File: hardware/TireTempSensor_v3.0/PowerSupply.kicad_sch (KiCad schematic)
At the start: 43 parts, among them IC3 TPS54202HDDCR, IC4 TPS54202HDDCR, Q1 FQT3P20TF, T10 TP_+5V, T11 TP_+5V, T12 TP_+5V, T13 TP_+5V, T14 TP_+3.3V, T15 TP_+2.6V, T8 TP_VCC, U2 MIC5306-2.6YD5-TR

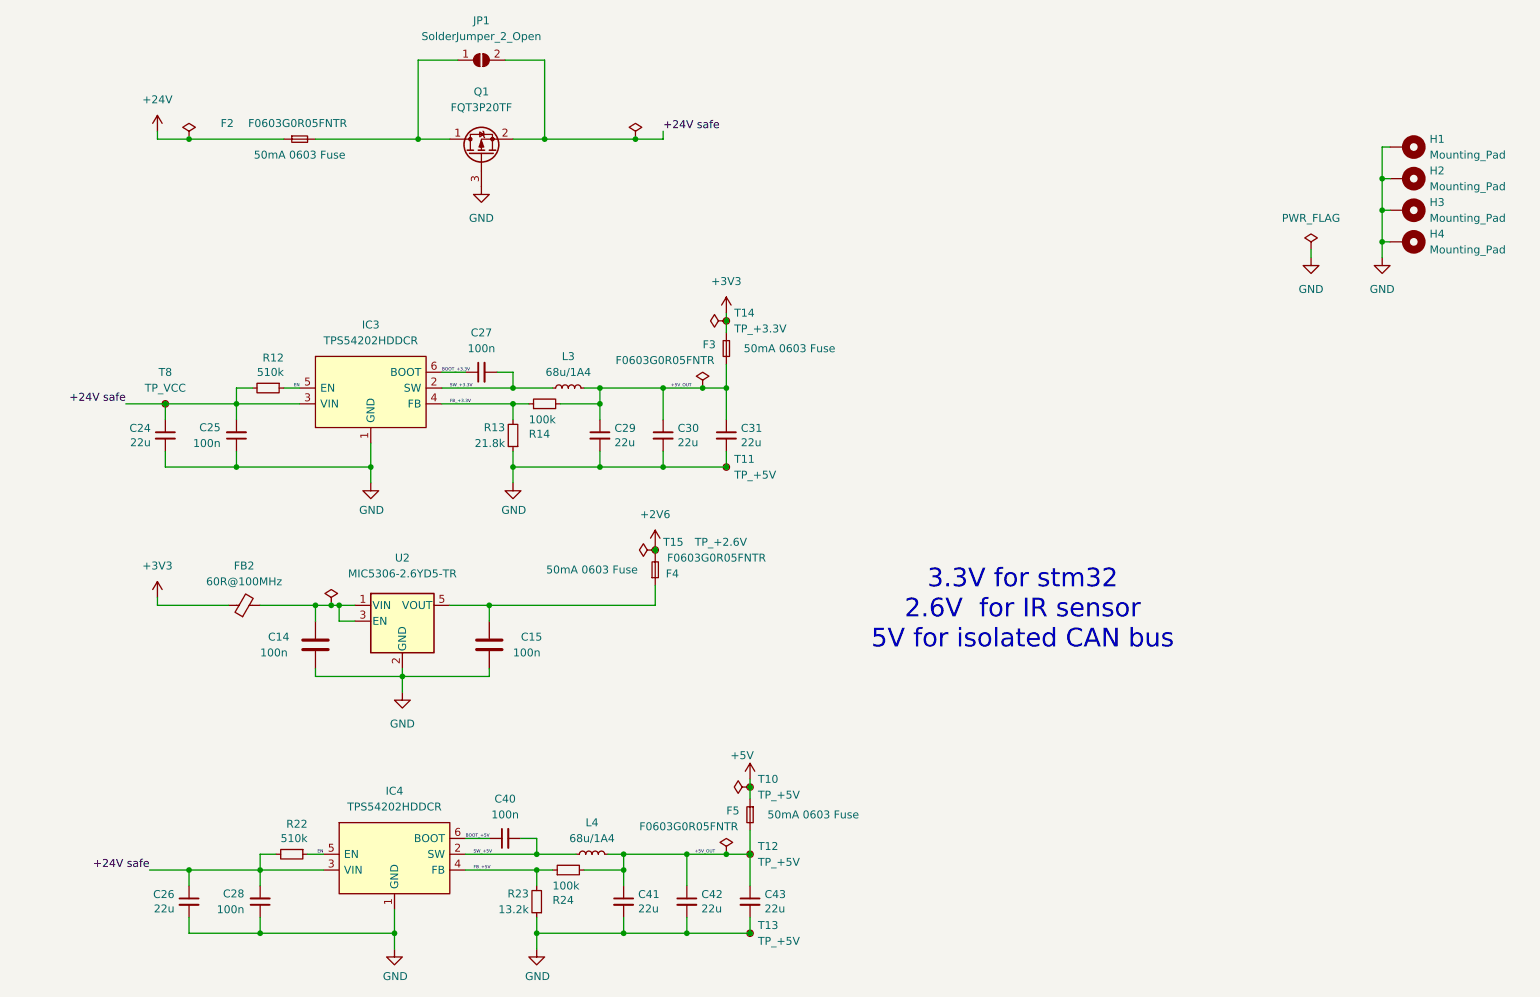
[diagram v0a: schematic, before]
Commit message: Piotruś prosił :3
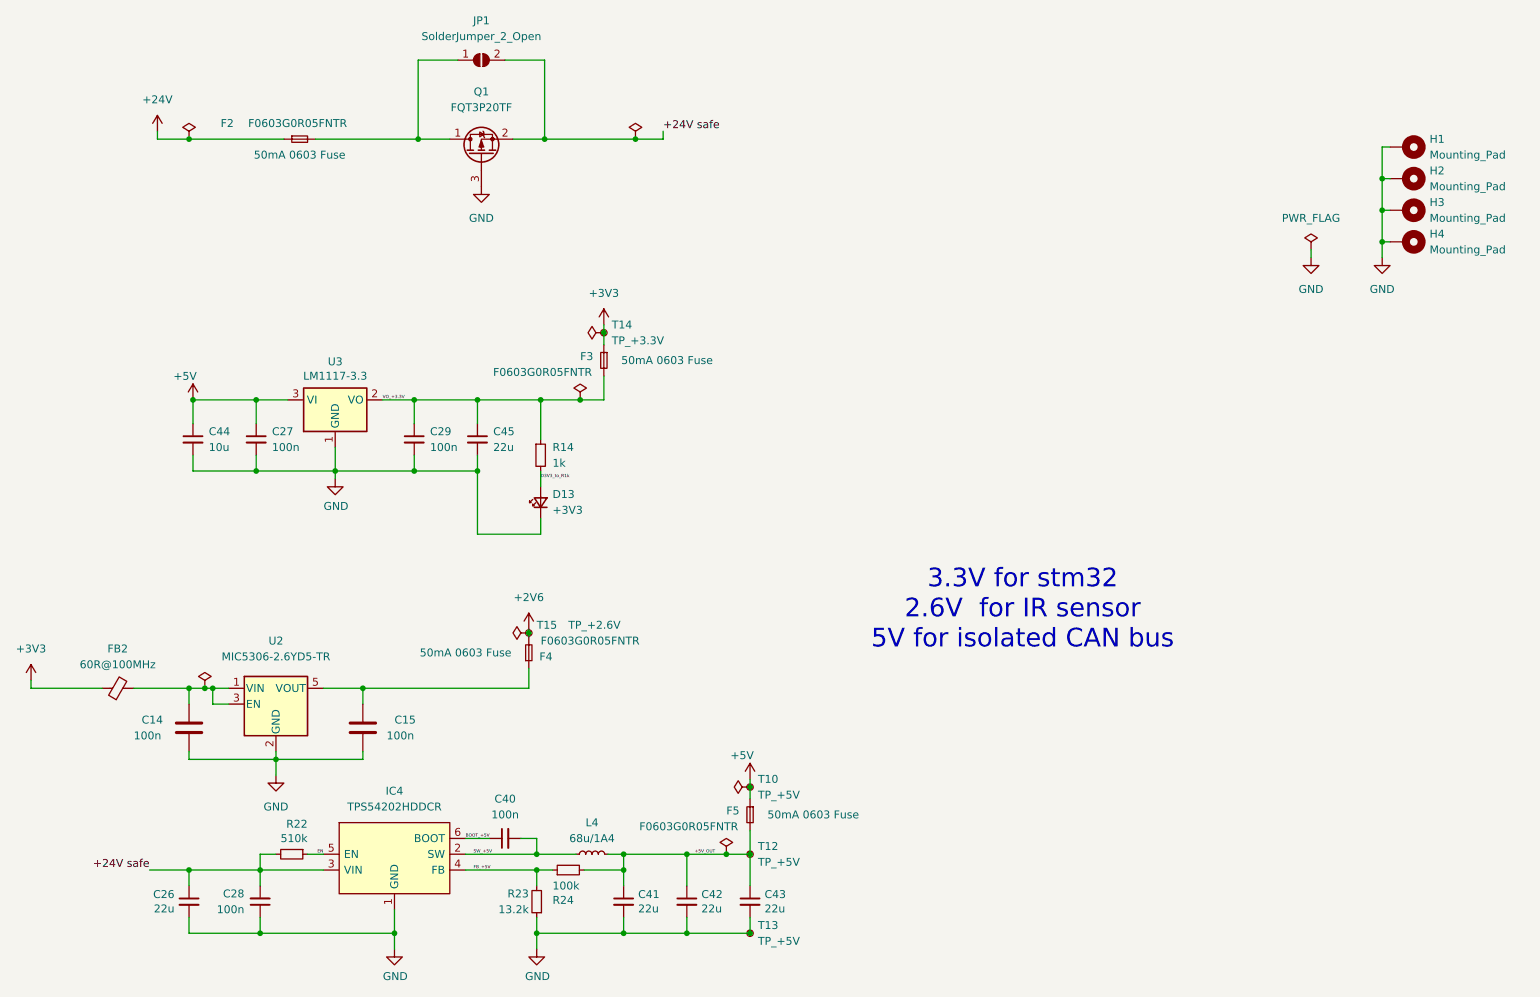
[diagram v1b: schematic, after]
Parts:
- removed C24, C30, C31: 22u, Capacitor_SMD:C_0805_2012Metric_Pad1.18x1.45mm_HandSolder, symbol Device:C_Small
- removed C25: 100n, Capacitor_SMD:C_0603_1608Metric_Pad1.08x0.95mm_HandSolder, symbol Device:C_Small
- removed IC3: TPS54202HDDCR, Package_TO_SOT_SMD:SOT-23-6_Handsoldering, symbol SamacsysNew:TPS54202HDDCR
- removed L3: 68u/1A4, Inductor_SMD:L_TDK_VLS6045EX_VLS6045AF, symbol Samacsys_kicad_sym:SRR4028-271Y
- removed R12: 510k, Resistor_SMD:R_0603_1608Metric_Pad0.98x0.95mm_HandSolder, symbol Device:R_Small
- removed R13: 21.8k, Resistor_SMD:R_0603_1608Metric_Pad0.98x0.95mm_HandSolder, symbol Device:R_Small
- removed T11: TP_+5V, TestPoint:TestPoint_Pad_1.0x1.0mm, symbol Connector:TestPoint_Small
- removed T8: TP_VCC, TestPoint:TestPoint_Pad_1.0x1.0mm, symbol Connector:TestPoint_Small
- added C44: 10u, Capacitor_SMD:C_0603_1608Metric_Pad1.08x0.95mm_HandSolder, symbol Device:C_Small
- added C45: 22u, Capacitor_SMD:C_0805_2012Metric_Pad1.18x1.45mm_HandSolder, symbol Device:C_Small
- added D13: +3V3, LED_SMD:LED_0603_1608Metric_Pad1.05x0.95mm_HandSolder, symbol Device:LED_Small
- added U3: LM1117-3.3, Package_TO_SOT_SMD:SOT-223-3_TabPin2, symbol Regulator_Linear:LM1117MP-3.3
- C29: value 22u -> 100n; footprint Capacitor_SMD:C_0805_2012Metric_Pad1.18x1.45mm_HandSolder -> Capacitor_SMD:C_0603_1608Metric_Pad1.08x0.95mm_HandSolder; Manufacturer_Name MCASH21GCC7684MTCA1J -> (none); Manufacturer_Part_Number CL21A107MQYNNWE -> (none); Mouser Part Number 810-C2012X5R1V226MAC -> (none); Mouser Price/Stock https://www.mouser.pl/ProductDetail/TDK/C2012X5R1V226M125AC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 -> https://www.mouser.pl/ProductDetail/Murata-Electronics/GRM0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
- R14: value 100k -> 1k; Manufacturer_Name -- -> (none); Manufacturer_Part_Number RT0603DRE07100KL -> (none); Mouser Part Number 603-RT0603DRE07100KL -> (none); Mouser Price/Stock https://www.mouser.pl/ProductDetail/KOA-Speer/RK73B1JTTD104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 -> https://www.mouser.pl/ProductDetail/Vishay-Dale/CRCW06031K0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
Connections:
- net BOOT_+3.3V is gone; now on net +5V: C27.1
- net SW_+3.3V is gone; now on net GND: C27.2
- net +5V: now also C44.1, U3.3 (VI)
- net +5V_OUT: no longer C29.1, F3.2, R14.2
- net GND: now also C44.2, C45.2, D13.1 (K), U3.1 (GND)
- net FB_+3.3V renamed VO_+3.3V
- net VO_+3.3V: now also C29.1, F3.2, C45.1, U3.2 (VO)
- new net D3V3_to_R1k: D13.2 (A), R14.2
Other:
- moved on the sheet: C14, C15, F3, F4, FB2, T14, T15, U2

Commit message: Poprawki, kontynuacja layoutu
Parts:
- Q1: footprint Mosfet:SOT-223-4-NFET -> Package_TO_SOT_SMD:SOT-223-3_TabPin2
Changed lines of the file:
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@@
 			)
 		)
-		(property "Footprint" "Mosfet:SOT-223-4-NFET"
+		(property "Footprint" "Package_TO_SOT_SMD:SOT-223-3_TabPin2"
 			(at 105.41 36.83 0)
 			(effects
@@
 			)
 		)
-		(property "Datasheet" "https://www.mouser.pl/ProductDetail/onsemi-Fairchild/FQT3P20TF?qs=k6rL%2Fc%252BPp3KKqr%252BK9hIArg%3D%3D"
+		(property "Datasheet" "https://www.mouser.pl/ProductDetail/Diodes-Incorporated/ZVP2120GTA?qs=xZ%2FP%252Ba9zWqYgxv%2FYfJ%252BkQg%3D%3D"
 			(at 107.95 41.91 0)
 			(effects

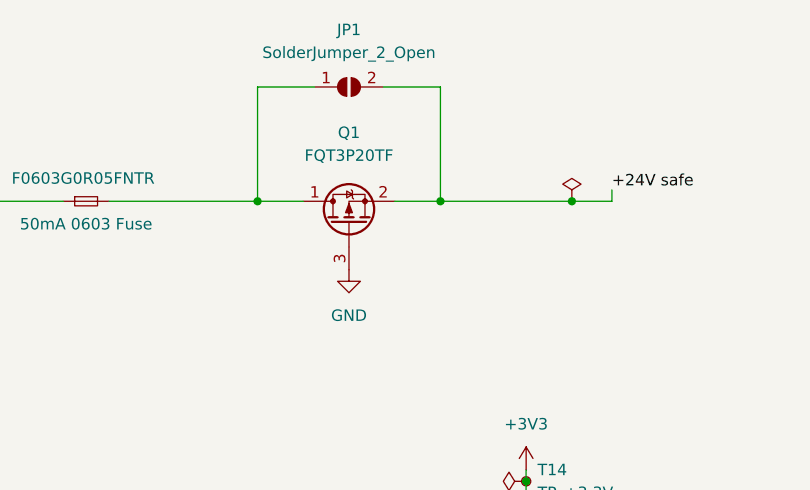
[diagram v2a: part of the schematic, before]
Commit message: Propozycja layoutu na spotkanie
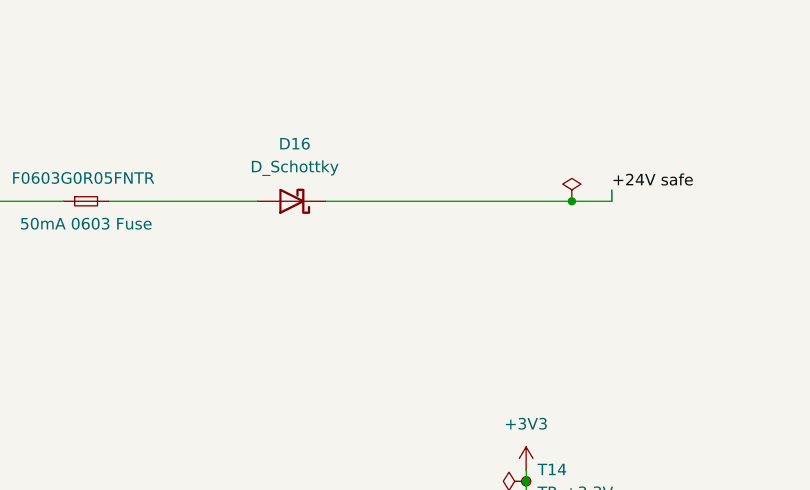
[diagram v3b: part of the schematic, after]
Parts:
- removed JP1: SolderJumper_2_Open, Jumper:SolderJumper-2_P1.3mm_Open_TrianglePad1.0x1.5mm, symbol Jumper:SolderJumper_2_Open
- removed Q1: FQT3P20TF, Package_TO_SOT_SMD:SOT-223-3_TabPin2, symbol Device:Q_PMOS_DSG
- added D16: D_Schottky, Diode_SMD:D_SOD-882D, symbol Device:D_Schottky
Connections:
- net +24V safe: now also D16.1 (K)
- net at F2.2: now also D16.2 (A)
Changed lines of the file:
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@@
 	)
 	(junction
-		(at 118.11 39.37)
-		(diameter 0)
-		(color 0 0 0 0)
-	)
-	(junction
 		(at 151.13 154.305)
 		(diameter 0)
@@
 	)
 	(junction
-		(at 97.79 39.37)
-		(diameter 0)
-		(color 0 0 0 0)
-	)
-	(junction
 		(at 151.13 167.005)
 		(diameter 0)
@@
 	(wire
 		(pts
-			(xy 118.11 26.67) (xy 118.11 39.37)
-		)
-		(stroke
-			(width 0)
-			(type default)
-		)
-	)
-	(wire
-		(pts
-			(xy 111.76 26.67) (xy 118.11 26.67)
-		)
-		(stroke
-			(width 0)
-			(type default)
-		)
-	)
-	(wire
-		(pts
 			(xy 116.84 154.305) (xy 123.19 154.305)
 		)
@@
 	(wire
 		(pts
-			(xy 97.79 39.37) (xy 102.87 39.37)
+			(xy 127.635 70.485) (xy 127.635 72.39)
 		)
 		(stroke
@@
 	(wire
 		(pts
-			(xy 127.635 70.485) (xy 127.635 72.39)
+			(xy 105.41 39.37) (xy 132.715 39.37)
 		)
 		(stroke
@@
 	(wire
 		(pts
-			(xy 97.79 26.67) (xy 104.14 26.67)
-		)
-		(stroke
-			(width 0)
-			(type default)
-		)
-	)
-	(wire
-		(pts
 			(xy 60.96 164.465) (xy 60.96 167.005)
 		)
@@
 	(wire
 		(pts
-			(xy 97.79 39.37) (xy 97.79 26.67)
-		)
-		(stroke
-			(width 0)
-			(type default)
-		)
-	)
-	(wire
-		(pts
 			(xy 60.96 137.795) (xy 60.96 139.065)
 		)
@@
 	(wire
 		(pts
-			(xy 118.11 39.37) (xy 132.715 39.37)
-		)
-		(stroke
-			(width 0)
-			(type default)
-		)
-	)
-	(wire
-		(pts
 			(xy 93.98 167.005) (xy 72.39 167.005)
 		)
@@
 	(wire
 		(pts
-			(xy 113.03 39.37) (xy 118.11 39.37)
-		)
-		(stroke
-			(width 0)
-			(type default)
-		)
-	)
-	(wire
-		(pts
 			(xy 252.73 55.88) (xy 252.73 58.42)
 		)
@@
 	)
 	(symbol
+		(lib_id "Device:D_Schottky")
+		(at 101.6 39.37 180)
+		(unit 1)
+		(exclude_from_sim no)
+		(in_bom yes)
+		(on_board yes)
+		(dnp no)
+		(fields_autoplaced yes)
+		(property "Reference" "D16"
+			(at 101.9175 33.02 0)
+			(effects
+				(font
+					(size 1.27 1.27)
+				)
+			)
+		)
+		(property "Value" "D_Schottky"
+			(at 101.9175 35.56 0)
+			(effects
+				(font
+					(size 1.27 1.27)
+				)
+			)
+		)
+		(property "Footprint" "Diode_SMD:D_SOD-882D"
+			(at 101.6 39.37 0)
+			(effects
+				(font
+					(size 1.27 1.27)
+				)
+				(hide yes)
+			)
+		)
+		(property "Datasheet" "https://www.mouser.pl/ProductDetail/Nexperia/BAS70L315?qs=me8TqzrmIYUQykHMkkfEBQ%3D%3D"
+			(at 101.6 39.37 0)
+			(effects
+				(font
+					(size 1.27 1.27)
+				)
+				(hide yes)
+			)
+		)
+		(property "Description" "Schottky diode"
+			(at 101.6 39.37 0)
+			(effects
+				(font
+					(size 1.27 1.27)
+				)
+				(hide yes)
+			)
+		)
+		(pin "2"
+		)
+		(pin "1"
+		)
+		(instances
+			(project "TireTempSensor_v2.0"
+				(path "/6e95e1be-fdd6-40ae-a4f8-5c53e6058d6c/0f13de77-3258-490a-9a0b-6a199964636d"
+					(reference "D16")
+					(unit 1)
+				)
+			)
+		)
+	)
+	(symbol
 		(lib_id "Device:C_Small")
 		(at 72.39 161.925 180)
@@
 	)
 	(symbol
-		(lib_id "Device:Q_PMOS_DSG")
-		(at 107.95 41.91 90)
-		(unit 1)
-		(exclude_from_sim no)
-		(in_bom yes)
-		(on_board yes)
-		(dnp no)
-		(fields_autoplaced yes)
-		(property "Reference" "Q1"
-			(at 107.95 31.75 90)
-			(effects
-				(font
-					(size 1.27 1.27)
-				)
-			)
-		)
-		(property "Value" "FQT3P20TF"
-			(at 107.95 34.29 90)
-			(effects
-				(font
-					(size 1.27 1.27)
-				)
-			)
-		)
-		(property "Footprint" "Package_TO_SOT_SMD:SOT-223-3_TabPin2"
-			(at 105.41 36.83 0)
-			(effects
-				(font
-					(size 1.27 1.27)
-				)
-				(hide yes)
-			)
-		)
-		(property "Datasheet" "https://www.mouser.pl/ProductDetail/Diodes-Incorporated/ZVP2120GTA?qs=xZ%2FP%252Ba9zWqYgxv%2FYfJ%252BkQg%3D%3D"
-			(at 107.95 41.91 0)
-			(effects
-				(font
-					(size 1.27 1.27)
-				)
-				(hide yes)
-			)
-		)
-		(property "Description" ""
-			(at 107.95 41.91 0)
-			(effects
-				(font
-					(size 1.27 1.27)
-				)
-			)
-		)
-		(pin "1"
-		)
-		(pin "2"
-		)
-		(pin "3"
-		)
-		(instances
-			(project ""
-				(path "/6e95e1be-fdd6-40ae-a4f8-5c53e6058d6c/0f13de77-3258-490a-9a0b-6a199964636d"
-					(reference "Q1")
-					(unit 1)
-				)
-			)
-		)
-	)
-	(symbol
 		(lib_id "Device:C_Small")
 		(at 111.76 151.765 90)
@@
 	)
 	(symbol
-		(lib_id "Jumper:SolderJumper_2_Open")
-		(at 107.95 26.67 0)
-		(unit 1)
-		(exclude_from_sim no)
-		(in_bom yes)
-		(on_board yes)
-		(dnp no)
-		(fields_autoplaced yes)
-		(property "Reference" "JP1"
-			(at 107.95 20.32 0)
-			(effects
-				(font
-					(size 1.27 1.27)
-				)
-			)
-		)
-		(property "Value" "SolderJumper_2_Open"
-			(at 107.95 22.86 0)
-			(effects
-				(font
-					(size 1.27 1.27)
-				)
-			)
-		)
-		(property "Footprint" "Jumper:SolderJumper-2_P1.3mm_Open_TrianglePad1.0x1.5mm"
-			(at 107.95 26.67 0)
-			(effects
-				(font
-					(size 1.27 1.27)
-				)
-				(hide yes)
-			)
-		)
-		(property "Datasheet" "~"
-			(at 107.95 26.67 0)
-			(effects
-				(font
-					(size 1.27 1.27)
-				)
-				(hide yes)
-			)
-		)
-		(property "Description" ""
-			(at 107.95 26.67 0)
-			(effects
-				(font
-					(size 1.27 1.27)
-				)
-			)
-		)
-		(pin "1"
-		)
-		(pin "2"
-		)
-		(instances
-			(project ""
-				(path "/6e95e1be-fdd6-40ae-a4f8-5c53e6058d6c/0f13de77-3258-490a-9a0b-6a199964636d"
-					(reference "JP1")
-					(unit 1)
-				)
-			)
-		)
-	)
-	(symbol
 		(lib_id "power:PWR_FLAG")
 		(at 147.32 154.305 0)
@@
 					(unit 1)
 				)
-			)
-		)
-	)
-	(symbol
-		(lib_id "power:GND")
-		(at 107.95 46.99 0)
-		(unit 1)
-		(exclude_from_sim no)
-		(in_bom yes)
-		(on_board yes)
-		(dnp no)
-		(property "Reference" "#PWR0123"
-			(at 107.95 53.34 0)
-			(effects
-				(font
-					(size 1.27 1.27)
-				)
-				(hide yes)
-			)
-		)
-		(property "Value" "GND"
-			(at 107.95 52.07 0)
-			(effects
-				(font
-					(size 1.27 1.27)
-				)
-			)
-		)
-		(property "Footprint" ""
-			(at 107.95 46.99 0)
-			(effects
-				(font
-					(size 1.27 1.27)
-				)
-				(hide yes)
-			)
-		)
-		(property "Datasheet" ""
-			(at 107.95 46.99 0)
-			(effects
-				(font
-					(size 1.27 1.27)
-				)
-				(hide yes)
-			)
-		)
-		(property "Description" ""
-			(at 107.95 46.99 0)
-			(effects
-				(font
-					(size 1.27 1.27)
-				)
-			)
-		)
-		(pin "1"
-		)
-		(instances
-			(project ""
-				(path "/6e95e1be-fdd6-40ae-a4f8-5c53e6058d6c/0f13de77-3258-490a-9a0b-6a199964636d"
-					(reference "#PWR0123")
-					(unit 1)
-				)
